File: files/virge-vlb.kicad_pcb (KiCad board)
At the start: 4 copper layers, 240.5 x 70.4 mm, 90 parts, among them J1 VLB_slot, J2 VGA, U1 74LS244, U2 27C020, U7 86C325, U8 7404, U9 7408, Y1 14.318MHz

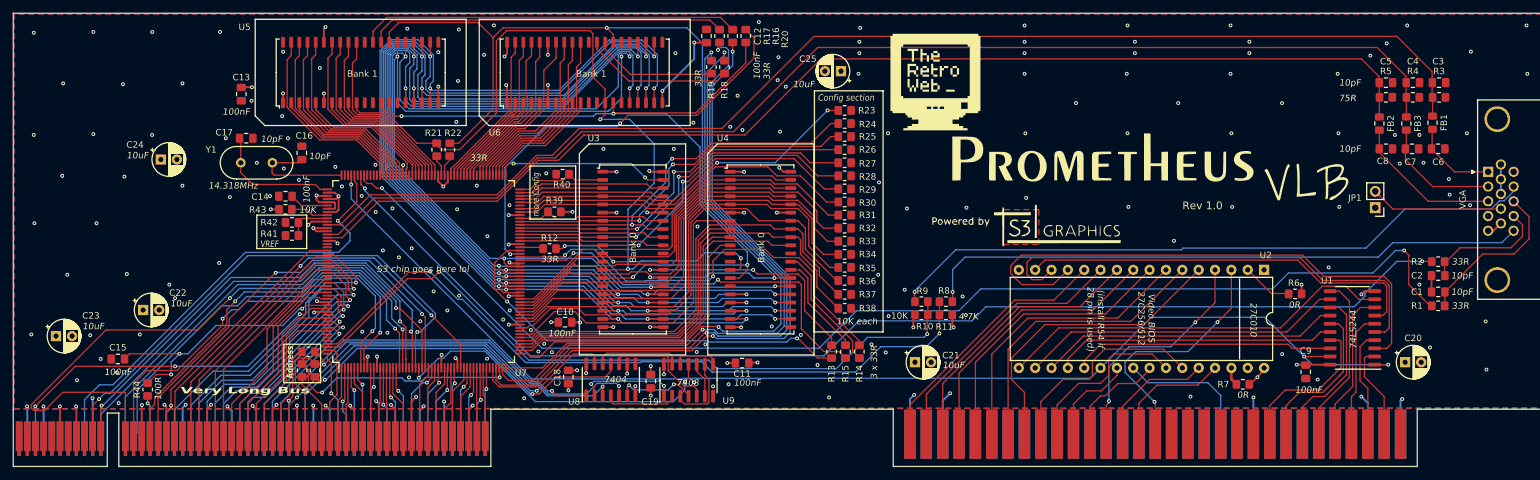
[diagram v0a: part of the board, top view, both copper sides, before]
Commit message: final changes for revision 1A
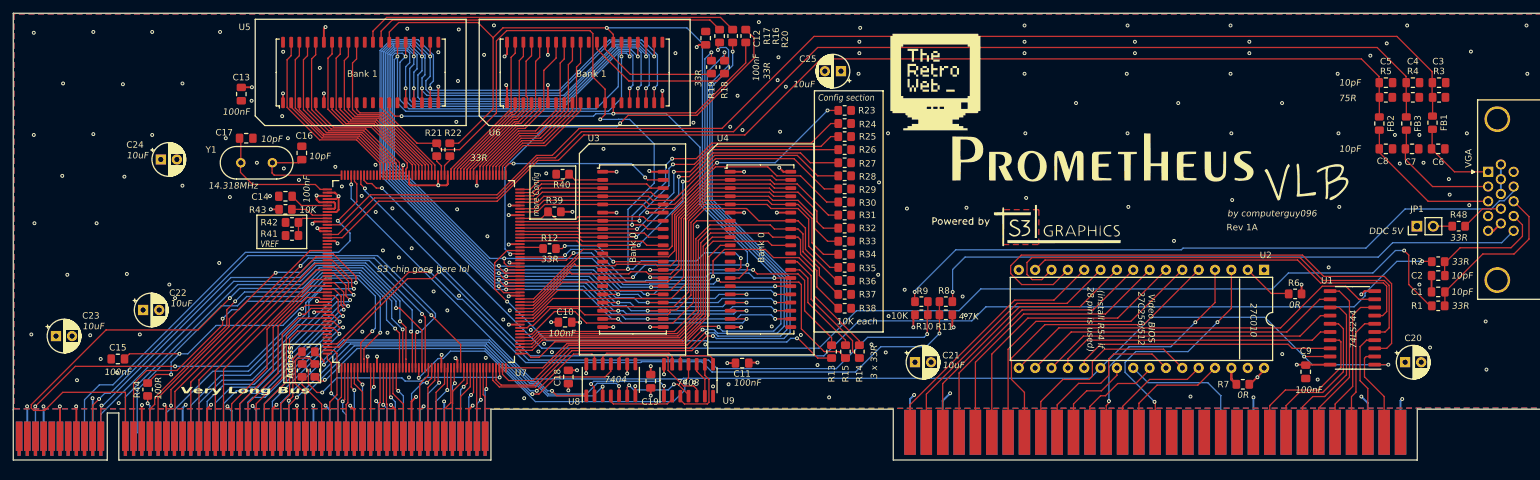
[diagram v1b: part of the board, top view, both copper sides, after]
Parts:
- added R48: 33R, Resistor_SMD:R_0805_2012Metric_Pad1.20x1.40mm_HandSolder, F.Cu at (255.9, 108.3)
- JP1: value Conn_01x02 -> DDC 5V
- moved JP1 7.08 mm to (249.4, 108.3), turned to 90 degrees
- moved C12 0.35 mm to (138.9, 79.1)
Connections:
- J2 pad 9: Net-(JP1-Pin_2) -> Net-(J2-Pad9)
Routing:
- net Net-(JP1-Pin_2): track 20.7 -> 2.95 mm
- net VCC: track 140.1 -> 128.9 mm
- net GND: track 153.6 -> 162.6 mm
- net Net-(J2-Pad9): track 0.00 -> 6.75 mm
- removed copper zone on F.Cu, net (none)
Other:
- board size 240.5 x 70.4 mm -> 240.5 x 69.4 mm
- board text added: "JLCJLCJLCJLC"
- board text added: "Rev 1A"
- board text added: "Special thanks to:"
- board text added: "by computerguy096"
- board text removed: "People who helped make this card:"
- board text removed: "Rev 1.0"
- board text removed: "computerguy096 (PCB)"
